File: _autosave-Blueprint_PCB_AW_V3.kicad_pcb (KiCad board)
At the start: 2 copper layers, 100 x 100 mm, 37 parts, among them J2 Conn_01x04_Pin, SW1 SW_Push, SW10 SW_Push, SW11 SW_Push, SW12 SW_Push, SW13 SW_Push, SW14 SW_Push, SW15 SW_Push, SW16 SW_Push, SW17 RotaryEncoder_Switch, SW2 SW_Push, SW3 SW_Push, SW4 SW_Push, SW5 SW_Push, SW6 SW_Push, SW7 SW_Push, SW8 SW_Push, SW9 SW_Push, U1 XIAO-RP2040-DIP

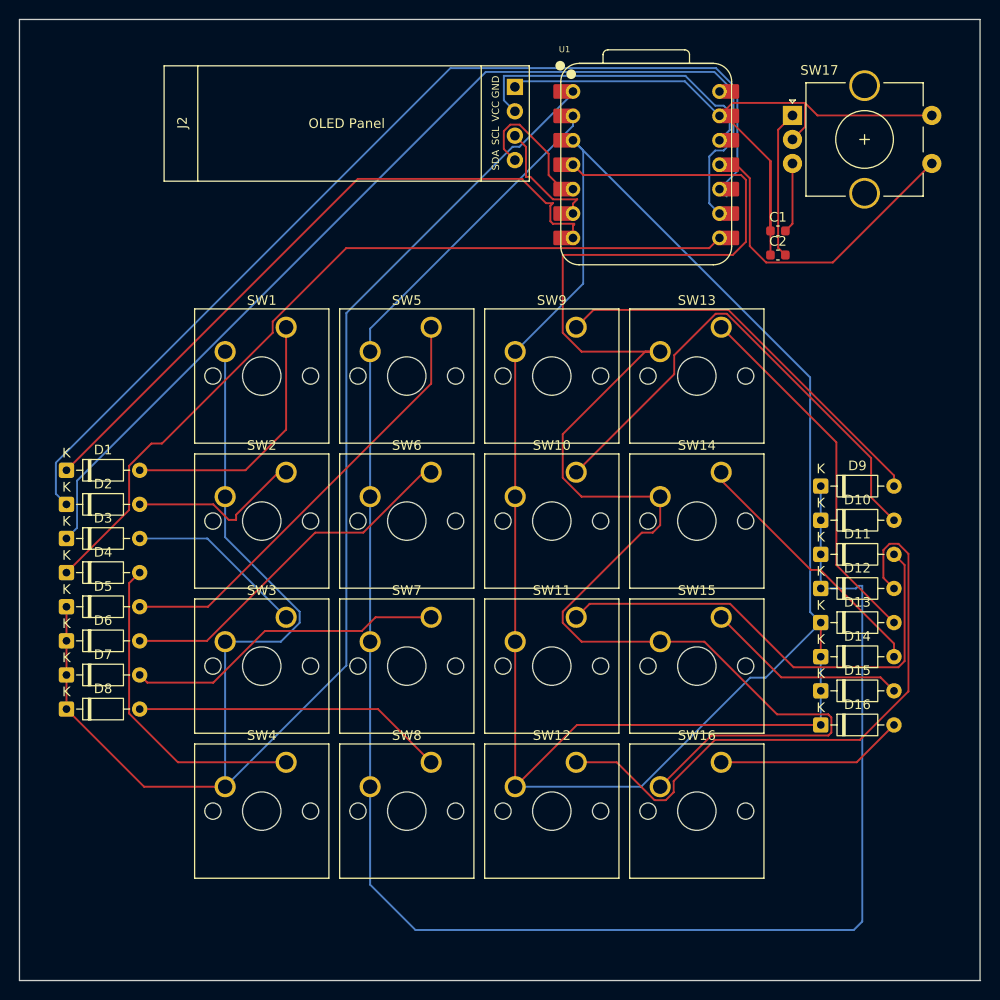
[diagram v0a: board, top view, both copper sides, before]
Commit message: Finished PCB
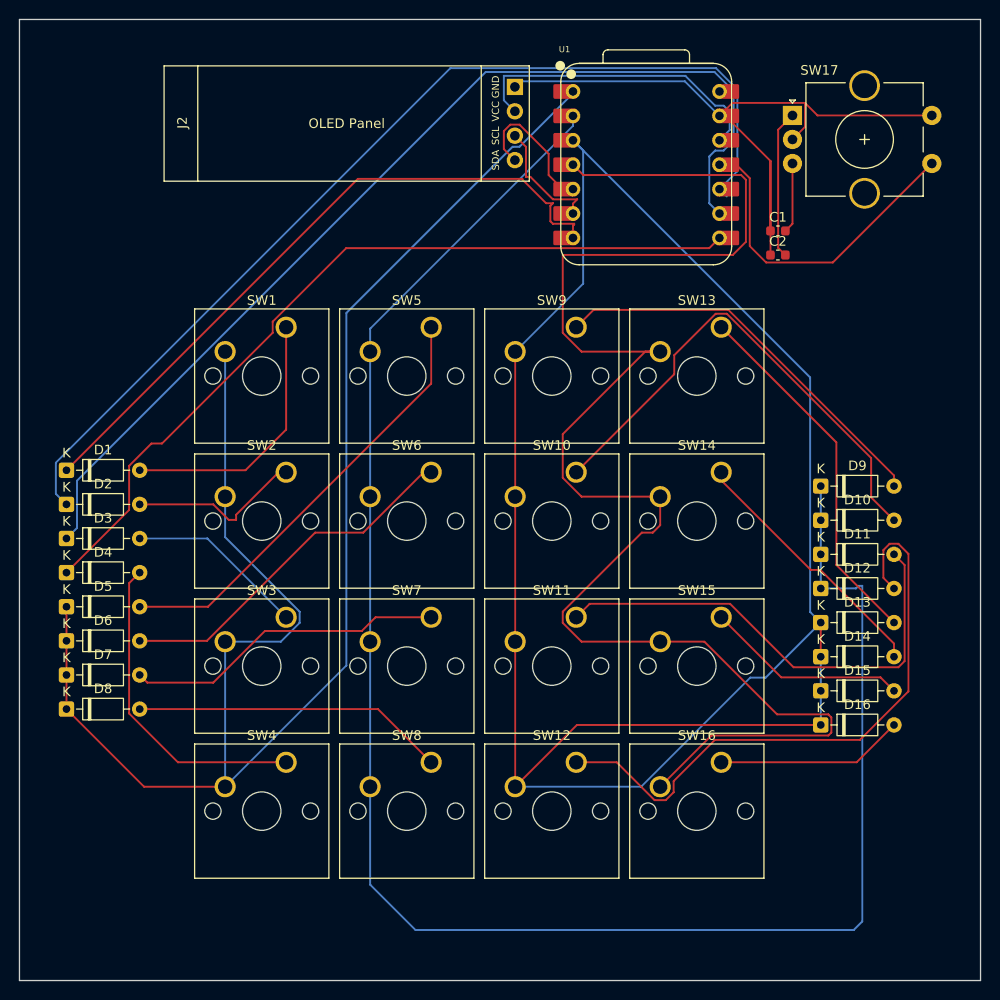
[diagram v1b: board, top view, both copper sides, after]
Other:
- outline, holes or cut-outs redrawn
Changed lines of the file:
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@@
 	)
 	(gr_line
-		(start 190.3095 14.478)
-		(end 190.3095 114.478)
+		(start 190.3605 14.478)
+		(end 190.3605 114.478)
 		(stroke
 			(width 0.05)
@@
 	(gr_line
 		(start 90.3605 14.478)
-		(end 190.3095 14.478)
+		(end 190.3605 14.478)
 		(stroke
 			(width 0.05)
